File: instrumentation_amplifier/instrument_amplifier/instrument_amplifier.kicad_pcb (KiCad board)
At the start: 2 copper layers, 72.9 x 41 mm, 20 parts, among them J1 Conn_01x06_Pin, U1 LM324, U2 LM324

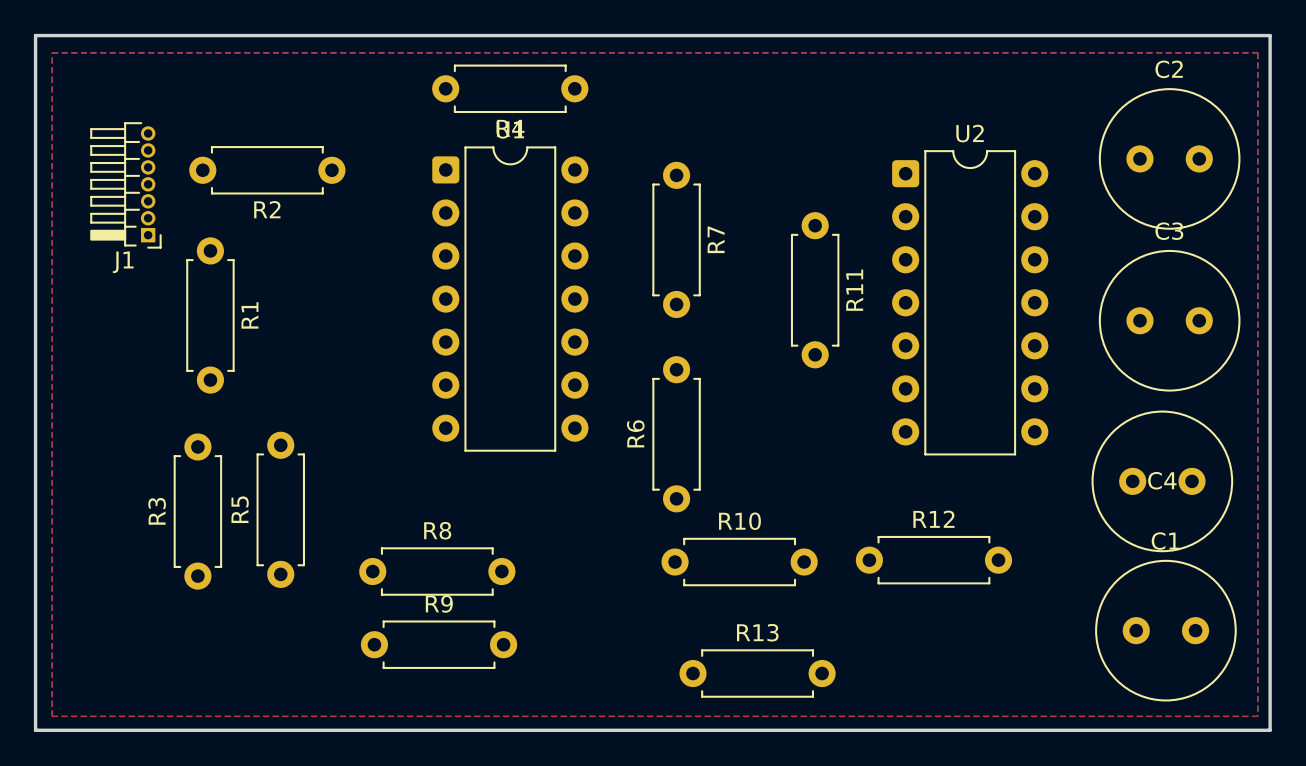
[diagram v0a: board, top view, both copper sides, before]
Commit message: final commit, ready to fab
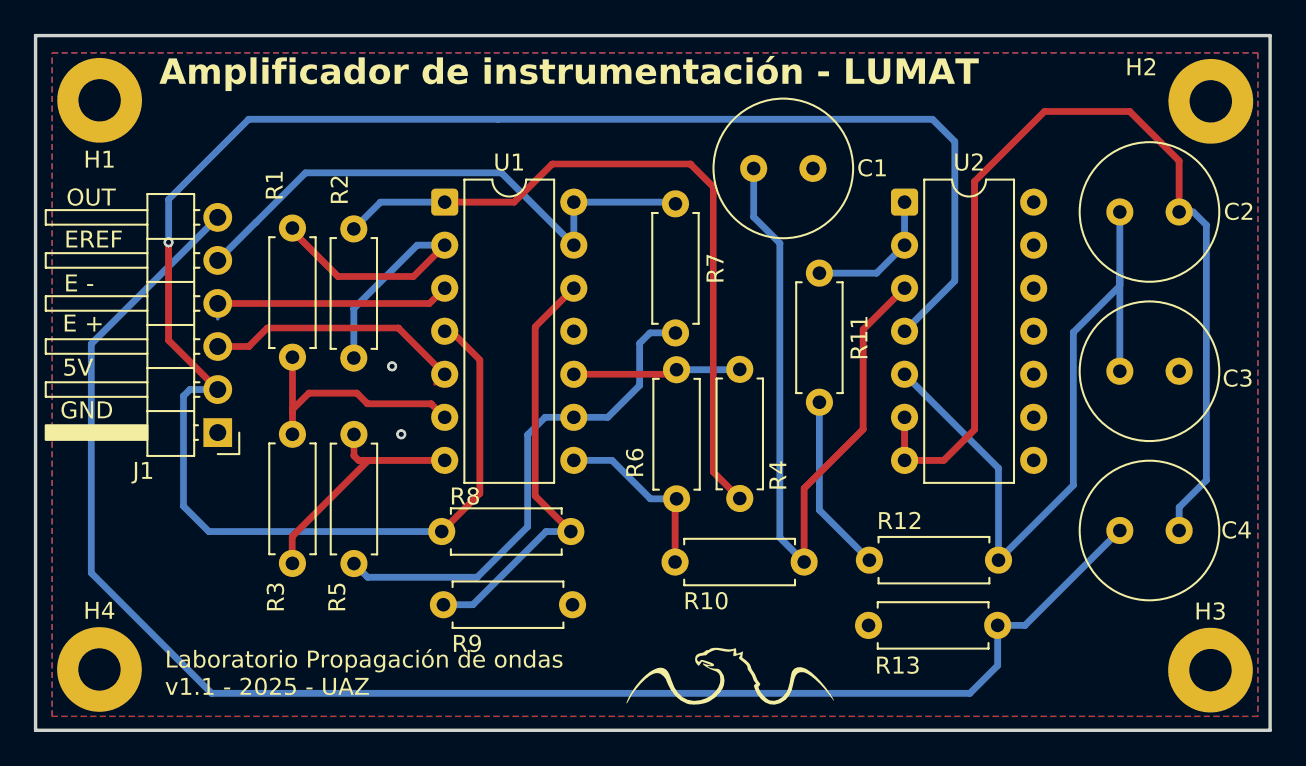
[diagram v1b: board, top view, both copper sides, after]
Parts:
- added G***: LOGO, LOGO, F.Cu at (91.7, 77.0)
- added H1: MountingHole_Pad, MountingHole:MountingHole_2.5mm_Pad, F.Cu at (54.8, 43.8)
- added H2: MountingHole_Pad, MountingHole:MountingHole_2.5mm_Pad, F.Cu at (120.4, 43.8)
- added H3: MountingHole_Pad, MountingHole:MountingHole_2.5mm_Pad, F.Cu at (120.4, 77.4)
- added H4: MountingHole_Pad, MountingHole:MountingHole_2.5mm_Pad, F.Cu at (54.8, 77.4)
- J1: footprint Connector_PinHeader_1.00mm:PinHeader_1x07_P1.00mm_Horizontal -> Connector_PinHeader_2.54mm:PinHeader_1x06_P2.54mm_Horizontal
- moved C1 35.4 mm to (93.4, 47.8)
- moved R4 19.2 mm to (92.6, 59.7), turned to -90 degrees
- moved J1 12.4 mm to (61.8, 63.4)
- moved R13 10.7 mm to (100.2, 74.8)
- moved R3 5.63 mm to (66.2, 71.1)
- moved R1 5.02 mm to (66.2, 51.3)
- moved R8 4.70 mm to (75.0, 69.2)
- moved R9 4.70 mm to (75.1, 73.5)
- moved R5 4.37 mm to (69.8, 71.1)
- moved R2 3.69 mm to (69.8, 51.4), turned to -90 degrees
- moved C2 3.35 mm to (115.0, 50.4)
- moved C3 3.21 mm to (115.0, 59.8)
- moved C4 3.00 mm to (115.0, 69.2)
- moved R11 2.81 mm to (97.3, 54.0)
- moved U1 1.90 mm to (75.2, 49.8)
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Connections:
- J1 pad 3: /E+ -> /E-
- J1 pad 4: /E- -> /E+
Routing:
- net +5V: track 0.00 -> 112.1 mm, vias 0 -> 1
- net /OUT_F: track 0.00 -> 93.1 mm
- net Net-(U2B--): track 0.00 -> 60.7 mm
- net Net-(U2A-+): track 0.00 -> 43.1 mm
- net Net-(U2B-+): track 0.00 -> 42.6 mm
- net Net-(R2-Pad1): track 0.00 -> 42.4 mm
- net /EREF: track 0.00 -> 33.5 mm
- net Net-(U1C--): track 0.00 -> 30.1 mm
- net Net-(U1D-+): track 0.00 -> 25.5 mm
- net Net-(U1A--): track 0.00 -> 20.9 mm
- net /E-: track 0.00 -> 15.8 mm
- net Net-(R3-Pad1): track 0.00 -> 15.2 mm
- net Net-(U1B--): track 0.00 -> 14.7 mm
- net /E+: track 0.00 -> 14.7 mm
- net /OUT: track 0.00 -> 10.8 mm
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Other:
- board text added: "5V"
- board text added: "Amplificador de instrumentación - LUMAT"
- board text added: "E +"
- board text added: "E -"
- board text added: "EREF"
- board text added: "GND"
- board text added: "Laboratorio Propagación de ondas v1.1 - 2025 - UAZ"
- board text added: "OUT"
